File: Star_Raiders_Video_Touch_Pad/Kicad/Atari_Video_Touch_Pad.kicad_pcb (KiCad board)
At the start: 2 copper layers, 50 x 120 mm, 8 parts, among them J1 DE9, SW1 FORE_VIEW, SW2 GAL_MAP, SW3 HYPERWARP, SW4 COMPUTER_ON/OFF, SW5 SHIELDS_ON/OFF

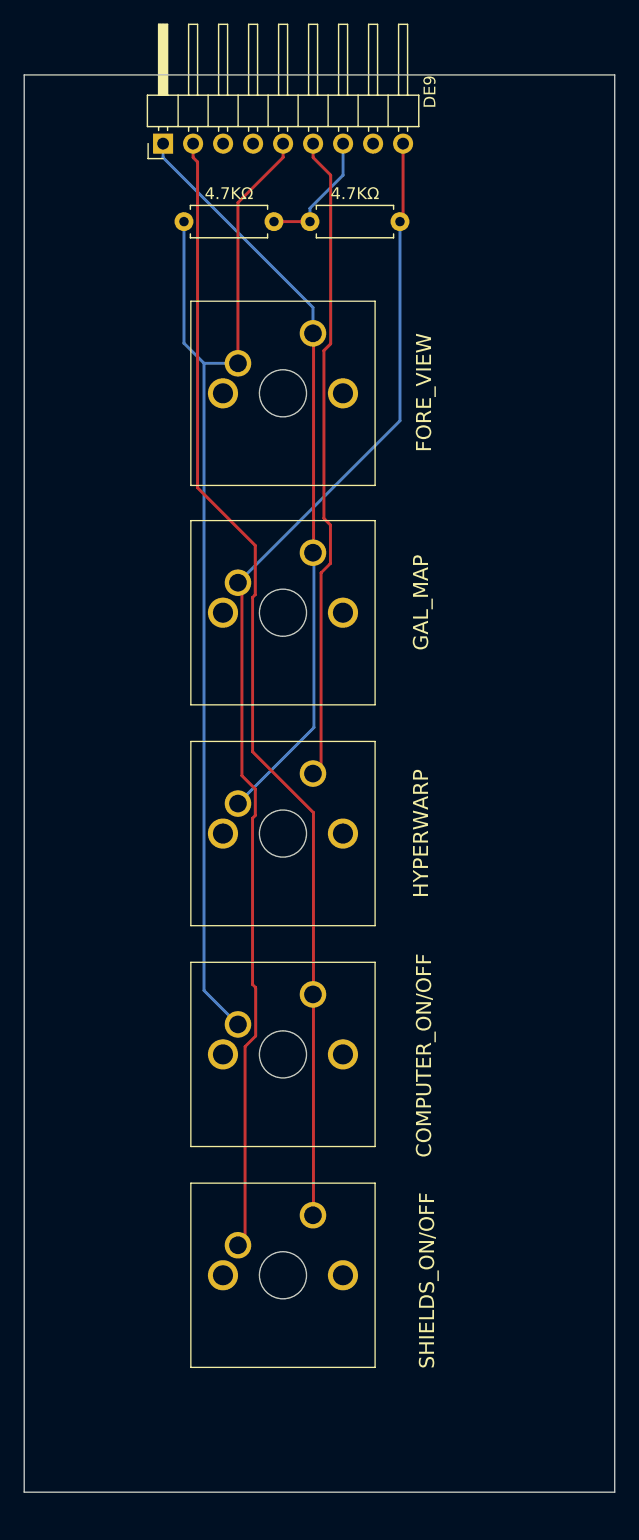
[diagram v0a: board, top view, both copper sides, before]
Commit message: Improved design (maybe?)
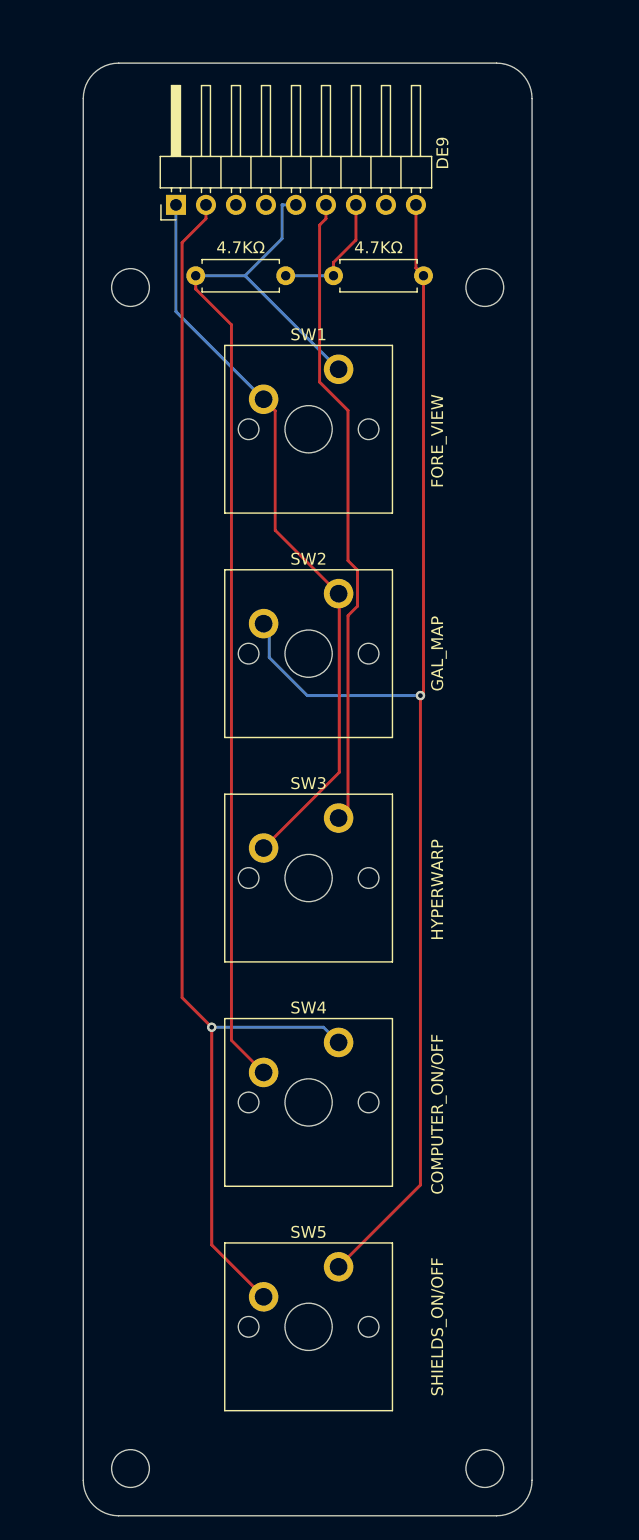
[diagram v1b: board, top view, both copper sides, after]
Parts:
- added H1: MountingHole, MountingHole:MountingHole_3.2mm_M3, F.Cu at (109.0, 148.0)
- added H2: MountingHole, MountingHole:MountingHole_3.2mm_M3, F.Cu at (139.0, 48.0)
- added H3: MountingHole, MountingHole:MountingHole_3.2mm_M3, F.Cu at (109.0, 48.0)
- added H4: MountingHole, MountingHole:MountingHole_3.2mm_M3, F.Cu at (139.0, 148.0)
- SW1, SW2, SW3, SW4, SW5: footprint MX1A-11NW:MX1A11NW -> PCM_Switch_Keyboard_Cherry_MX:SW_Cherry_MX_PCB_1.00u
- moved SW5 9.14 mm to (124.1, 136.0)
- moved SW4 8.91 mm to (124.1, 117.0)
- moved SW3 8.69 mm to (124.1, 98.0)
- moved SW2 8.48 mm to (124.1, 79.0)
- moved SW1 8.18 mm to (124.1, 60.0)
- moved J1 5.30 mm to (112.8, 41.0)
- moved R1 5.00 mm to (133.8, 47.0)
- moved R2 4.69 mm to (122.1, 47.0)
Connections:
- SW1 pad 1: /GREEN -> /BROWN
- SW1 pad 2: /BROWN -> /GREEN
- SW5 pad 1: /WHITE -> /RED
- SW5 pad 2: /RED -> /WHITE
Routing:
- net /RED: track 95.2 -> 107.4 mm, vias 0 -> 1
- net /WHITE: track 100.5 -> 110.4 mm, vias 0 -> 1
- net /BROWN: track 63.9 -> 62.8 mm
- net /BLUE: track 55.0 -> 54.1 mm
- net /GREEN: track 92.9 -> 93.7 mm
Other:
- board size 50 x 120 mm -> 38 x 123 mm
